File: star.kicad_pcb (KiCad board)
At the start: 2 copper layers, 76.1 x 72.4 mm, 43 parts, among them J1 Conn_01x05, J2 Conn_01x05, U1 74HCT1G125GW

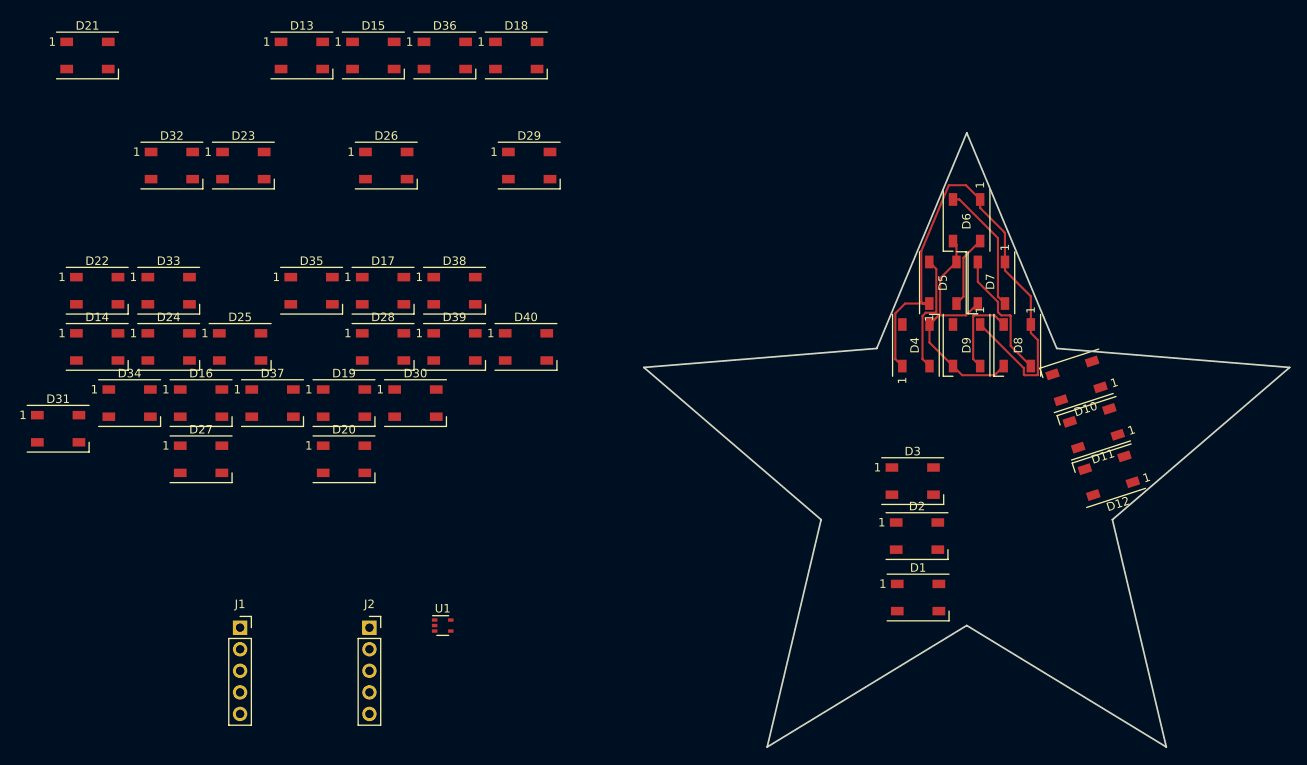
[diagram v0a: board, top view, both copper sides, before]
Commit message: Primer arreglo estelar
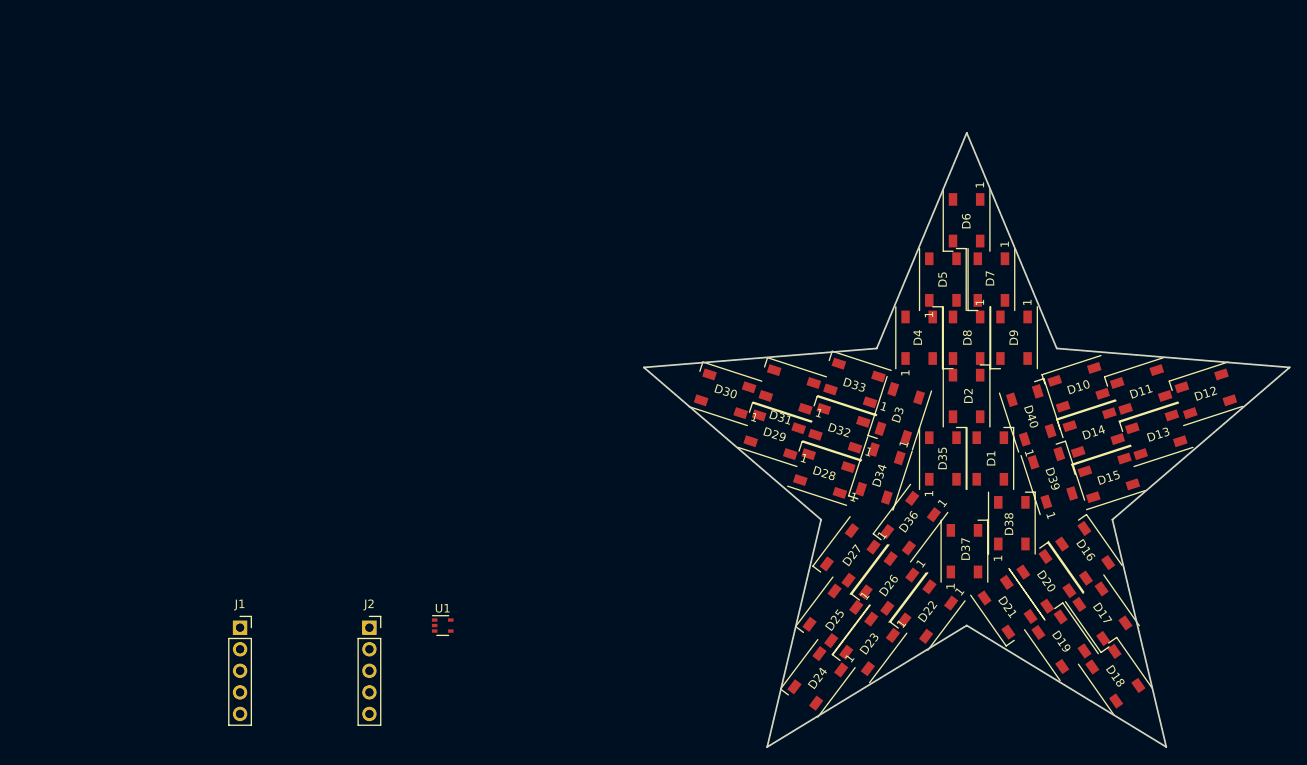
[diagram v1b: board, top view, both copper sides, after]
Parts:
- moved D21 126.4 mm to (174.0, 122.2), turned to 305 degrees
- moved D14 117.9 mm to (184.2, 101.6), turned to 198 degrees
- moved D13 110.1 mm to (191.5, 101.9), turned to 198 degrees
- moved D16 105.7 mm to (183.1, 115.8), turned to 125 degrees
- moved D22 104.9 mm to (164.6, 122.7), turned to 233 degrees
- moved D18 101.6 mm to (186.7, 130.3), turned to 125 degrees
- moved D15 99.9 mm to (185.9, 106.9), turned to 198 degrees
- moved D17 92.9 mm to (185.2, 122.9), turned to 305 degrees
- moved D23 92.8 mm to (157.7, 126.5), turned to 233 degrees
- moved D19 89.1 mm to (180.3, 126.2), turned to 125 degrees
- moved D34 88.8 mm to (159.0, 106.4), turned to 252 degrees
- moved D31 86.3 mm to (148.3, 96.5), turned to 162 degrees
- moved D24 85.9 mm to (151.6, 130.6), turned to 233 degrees
- moved D32 84.5 mm to (154.2, 101.1), turned to 162 degrees
- moved D20 84.0 mm to (178.6, 119.1), turned to 125 degrees
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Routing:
- net +5V: track 64.0 -> 0.00 mm
- net GND: track 30.9 -> 0.00 mm
- net Net-(D7-Pad2): track 15.5 -> 0.00 mm
- net Net-(D6-Pad2): track 15.2 -> 0.00 mm
- net Net-(D4-Pad2): track 14.3 -> 0.00 mm
- net Net-(D8-Pad2): track 10.3 -> 0.00 mm
- net Net-(D5-Pad2): track 8.52 -> 0.00 mm
